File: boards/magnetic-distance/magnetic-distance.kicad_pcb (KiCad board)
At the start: 2 copper layers, 23 x 19.5 mm, 7 parts, among them J1 CONN_02X03, M3 MountingHole_3.2mm_M3, U1 DS9638, U2 AS5304

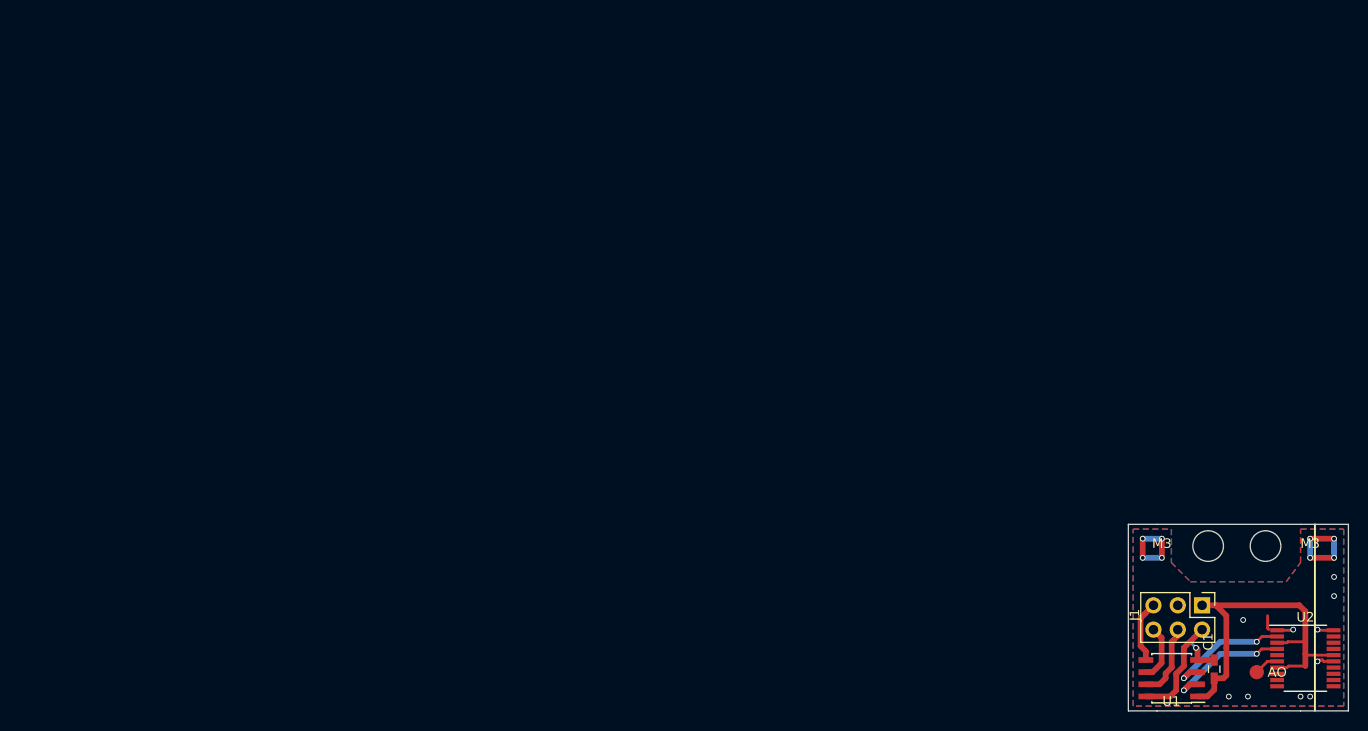
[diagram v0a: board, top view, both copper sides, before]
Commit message: [docs] export all board layouts
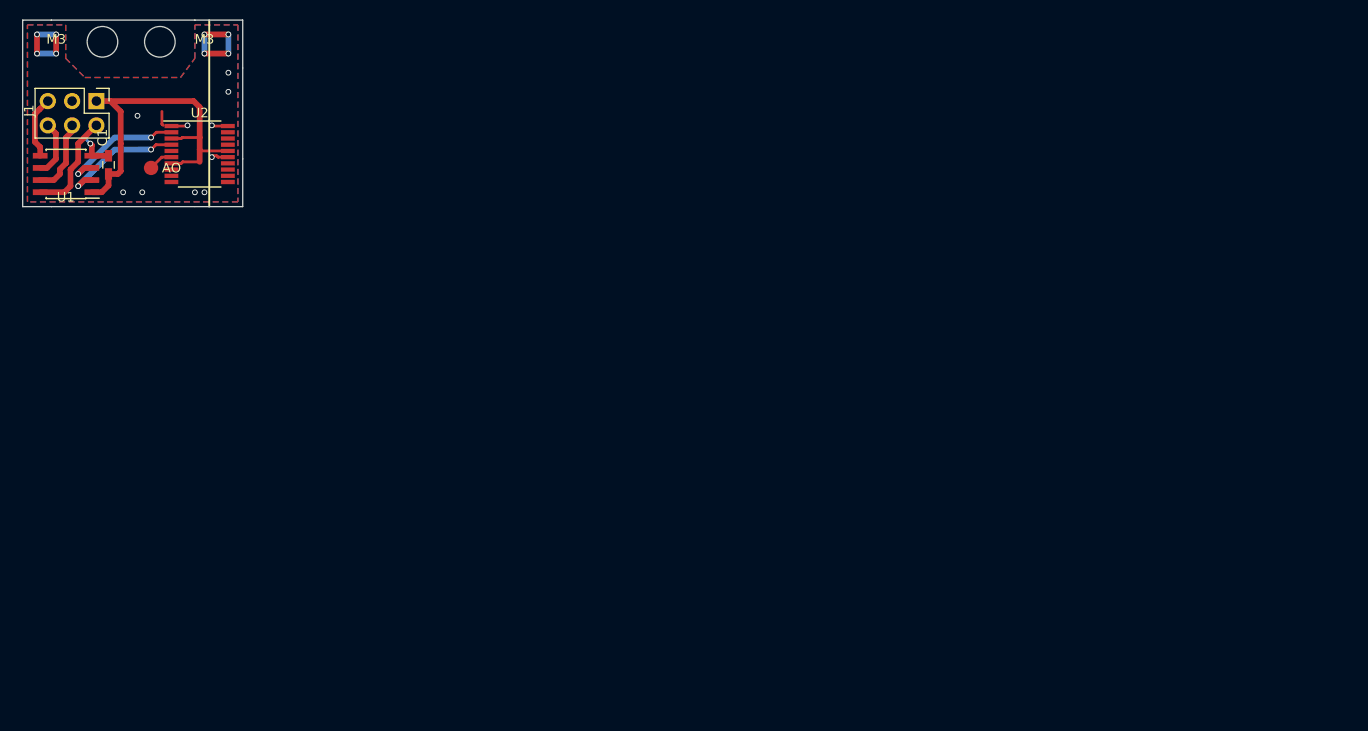
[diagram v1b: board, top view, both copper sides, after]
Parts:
- moved J1 127.0 mm to (64.1, 48.3)
- moved AO 127.0 mm to (69.8, 55.2)
- moved C1 127.0 mm to (65.4, 54.9)
- moved U2 127.0 mm to (74.9, 53.8)
- moved M3 127.0 mm to (70.8, 42.1)
- moved M3 127.0 mm to (64.8, 42.1)
- moved U1 127.0 mm to (61.0, 55.9)
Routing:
- net (no net): track 17.0 -> 18.5 mm
- net /GND: track 10.6 -> 9.10 mm
